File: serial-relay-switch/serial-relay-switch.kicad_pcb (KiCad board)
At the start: 2 copper layers, 41.9 x 31.8 mm, 58 parts, among them J10 Conn_01x01, J11 Conn_01x01, J12 Conn_01x01, J13 Conn_01x01, J14 Conn_01x01, J15 Conn_01x01, J16 Conn_01x01, J17 Conn_01x01, J18 Conn_01x01, J2 2501551-4, J3 Conn_01x01, J4 Conn_01x01, J5 Conn_01x01, J6 Conn_01x01, J7 Conn_01x01, J8 Conn_01x01, J9 Conn_01x01, U1 74LS166, U2 ISL8488E, U3 74LVC1G08, U4 ISL8488E

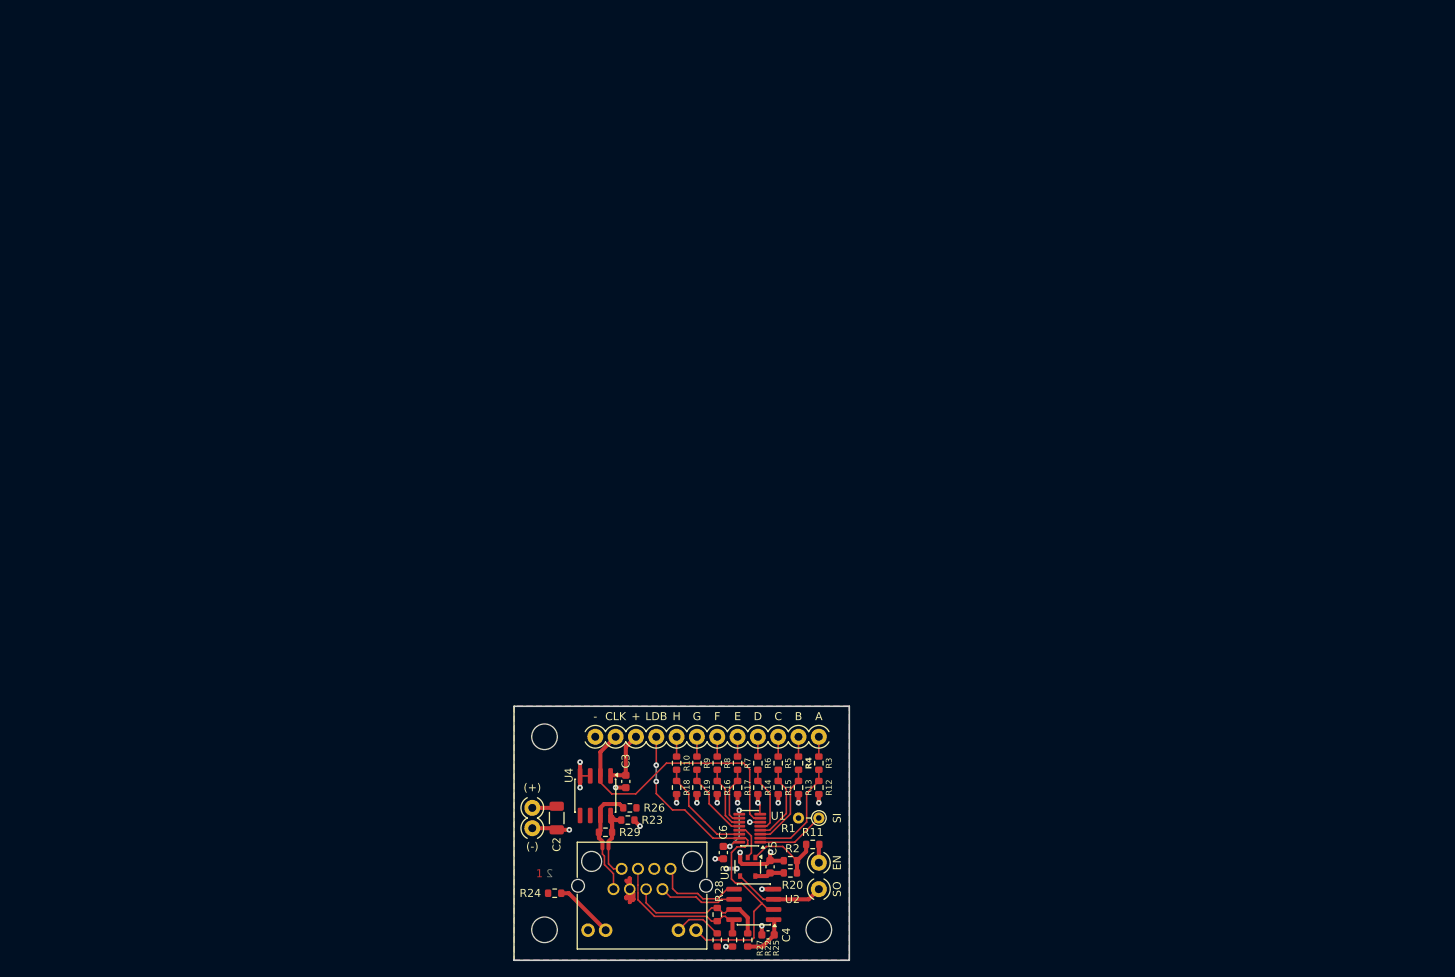
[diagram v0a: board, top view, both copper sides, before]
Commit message: [rs] Mostly complete preliminary PCB placement
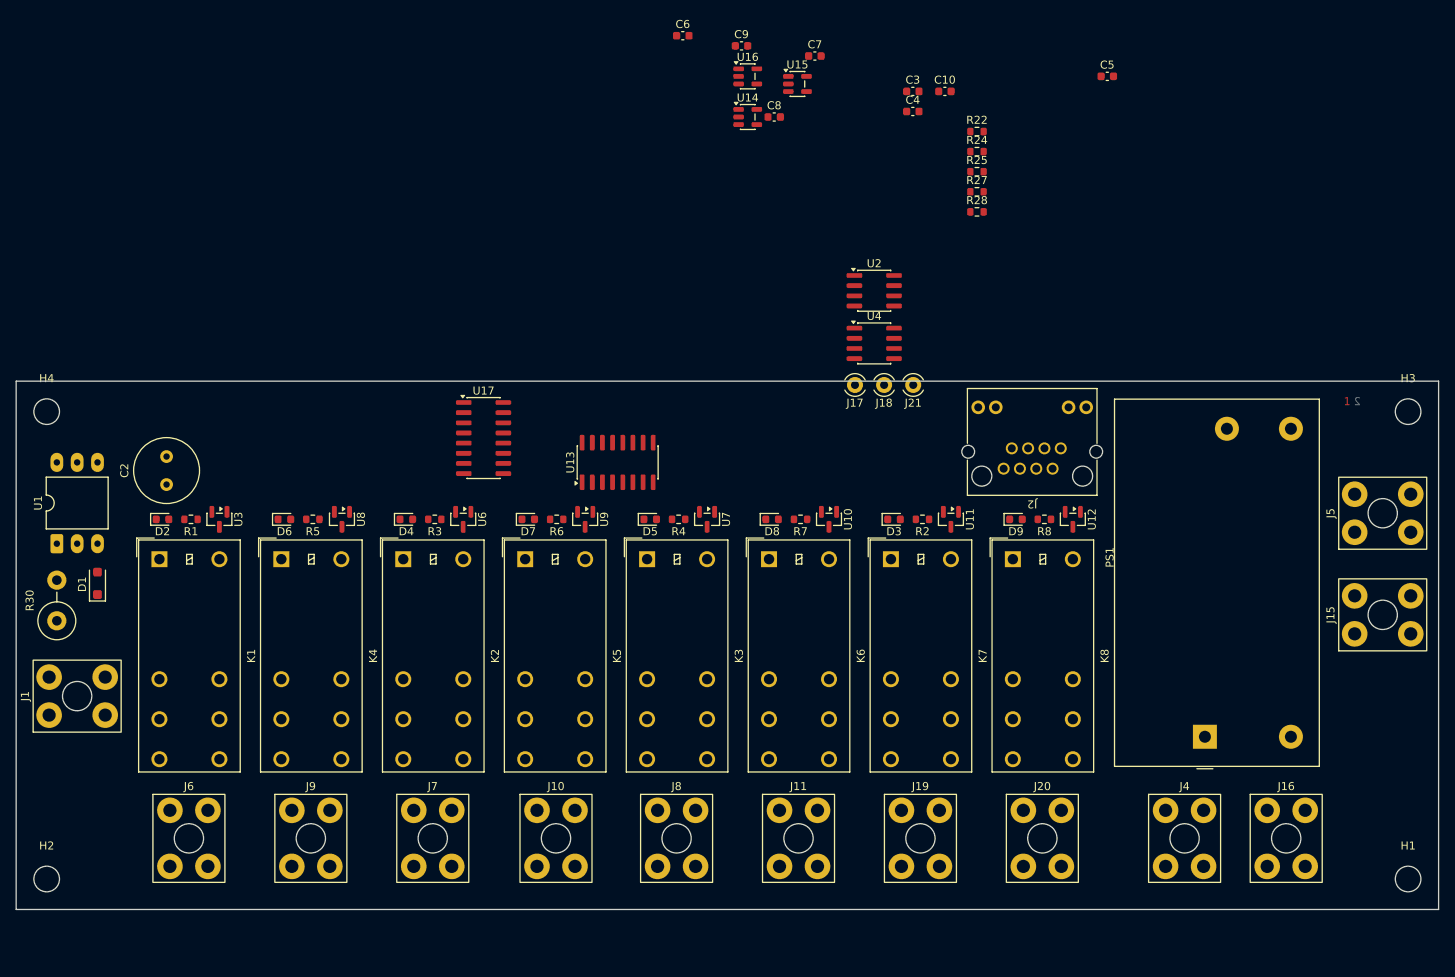
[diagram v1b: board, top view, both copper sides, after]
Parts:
- removed J12, J13, J14, J3: Conn_01x01, CUSTOM:Pin_D1.0mm
- removed R10, R11, R9: 1k, Resistor_SMD:R_0603_1608Metric
- removed R12, R13, R14, R15, R16, R17, R18, R19, R20, R23, R26: 10k, Resistor_SMD:R_0603_1608Metric
- removed R29: 120, Resistor_SMD:R_0603_1608Metric
- added C10: 0.1uF, Capacitor_SMD:C_0603_1608Metric, F.Cu at (153.9, 6.39)
- added C7: 0.1uF, Capacitor_SMD:C_0603_1608Metric, F.Cu at (137.6, 1.97)
- added C8: 0.1uF, Capacitor_SMD:C_0603_1608Metric, F.Cu at (132.5, 9.59)
- added C9: 0.1uF, Capacitor_SMD:C_0603_1608Metric, F.Cu at (128.4, 0.70)
- added D1: 1N4148, Diode_SMD:D_SOD-123F, F.Cu at (47.9, 67.9)
- added D2: LED, LED_SMD:LED_0603_1608Metric, F.Cu at (56.1, 59.9)
- added D3: LED, LED_SMD:LED_0603_1608Metric, F.Cu at (147.5, 59.9)
- added D4: LED, LED_SMD:LED_0603_1608Metric, F.Cu at (86.5, 59.9)
- added D5: LED, LED_SMD:LED_0603_1608Metric, F.Cu at (117.0, 59.9)
- added D6: LED, LED_SMD:LED_0603_1608Metric, F.Cu at (71.3, 59.9)
- added D7: LED, LED_SMD:LED_0603_1608Metric, F.Cu at (101.8, 59.9)
- added D8: LED, LED_SMD:LED_0603_1608Metric, F.Cu at (132.3, 59.9)
- added D9: LED, LED_SMD:LED_0603_1608Metric, F.Cu at (162.7, 59.9)
- added H4: MountingHole, MountingHole:MountingHole_3.2mm_M3, F.Cu at (41.6, 46.4)
- added J1: Screw_Terminal_01x01, CUSTOM:8195, F.Cu at (45.4, 82.0)
- added J19: Screw_Terminal_01x01, CUSTOM:8195, F.Cu at (150.8, 99.8)
- added J20: Screw_Terminal_01x01, CUSTOM:8195, F.Cu at (166.0, 99.8)
- added J21: Conn_01x01, CUSTOM:Pin_D1.0mm, F.Cu at (149.9, 43.1)
- added K1: G2RL-1-E, Relay_THT:Relay_SPDT_Omron_G2RL-1-E, F.Cu at (55.7, 64.9)
- added K2: G2RL-1-E, Relay_THT:Relay_SPDT_Omron_G2RL-1-E, F.Cu at (86.2, 64.9)
- added K3: G2RL-1-E, Relay_THT:Relay_SPDT_Omron_G2RL-1-E, F.Cu at (116.6, 64.9)
- added K4: G2RL-1-E, Relay_THT:Relay_SPDT_Omron_G2RL-1-E, F.Cu at (70.9, 64.9)
- added K5: G2RL-1-E, Relay_THT:Relay_SPDT_Omron_G2RL-1-E, F.Cu at (101.4, 64.9)
- added K6: G2RL-1-E, Relay_THT:Relay_SPDT_Omron_G2RL-1-E, F.Cu at (131.9, 64.9)
- added K7: G2RL-1-E, Relay_THT:Relay_SPDT_Omron_G2RL-1-E, F.Cu at (147.1, 64.9)
- added K8: G2RL-1-E, Relay_THT:Relay_SPDT_Omron_G2RL-1-E, F.Cu at (162.4, 64.9)
- added PS1: IRM-10-5, Converter_ACDC:Converter_ACDC_MeanWell_IRM-10-xx_THT, F.Cu at (186.4, 87.1)
- added R30: 100k, Resistor_THT:R_Axial_DIN0414_L11.9mm_D4.5mm_P5.08mm_Vertical, F.Cu at (42.9, 72.6)
- added U10: SZNUD3124LT1G, Package_TO_SOT_SMD:SOT-23, F.Cu at (139.4, 59.9)
- added U11: SZNUD3124LT1G, Package_TO_SOT_SMD:SOT-23, F.Cu at (154.6, 59.9)
- added U12: SZNUD3124LT1G, Package_TO_SOT_SMD:SOT-23, F.Cu at (169.8, 59.9)
- added U13: 74HCT595, Package_SO:SOIC-16_3.9x9.9mm_P1.27mm, F.Cu at (113.0, 52.8)
- added U14: 74LVC1G32, Package_TO_SOT_SMD:SOT-23-5, F.Cu at (129.2, 9.59)
- added U15: 74LVC1G08, Package_TO_SOT_SMD:SOT-23-5, F.Cu at (135.4, 5.46)
- added U16: 74LVC1G04, Package_TO_SOT_SMD:SOT-23-5, F.Cu at (129.2, 4.51)
- added U17: 74LS163, Package_SO:SOIC-16_3.9x9.9mm_P1.27mm, F.Cu at (96.2, 49.7)
- added U6: SZNUD3124LT1G, Package_TO_SOT_SMD:SOT-23, F.Cu at (93.7, 59.9)
- added U7: SZNUD3124LT1G, Package_TO_SOT_SMD:SOT-23, F.Cu at (124.1, 59.9)
- added U8: SZNUD3124LT1G, Package_TO_SOT_SMD:SOT-23, F.Cu at (78.5, 59.9)
- added U9: SZNUD3124LT1G, Package_TO_SOT_SMD:SOT-23, F.Cu at (108.9, 59.9)
- C2: footprint Capacitor_SMD:C_1206_3216Metric -> Capacitor_THT:C_Radial_D8.0mm_H7.0mm_P3.50mm
- J10, J11, J15, J16, J4, J5, J6, J7, J8, J9: value Conn_01x01 -> Screw_Terminal_01x01; footprint CUSTOM:Pin_D1.0mm -> CUSTOM:8195
- R1: value 10k -> 1k; footprint Resistor_THT:R_Axial_DIN0204_L3.6mm_D1.6mm_P2.54mm_Vertical -> Resistor_SMD:R_0603_1608Metric
- R2: value 10k -> 1k
- U1: value 74LS166 -> H11L1; footprint Package_SO:Texas_DYY0016A_TSOT-23-16_2x4.2mm_P0.5mm -> Package_DIP:DIP-6_W10.16mm_LongPads
- U3: value 74LVC1G08 -> SZNUD3124LT1G; footprint Package_SO:TSOP-5_1.65x3.05mm_P0.95mm -> Package_TO_SOT_SMD:SOT-23
- moved H3 125.9 mm to (211.8, 46.4)
- moved LAY1 116.9 mm to (204.1, 46.4)
- moved H1 109.4 mm to (211.8, 104.8)
- moved J15 109.0 mm to (208.6, 71.8)
- moved C5 107.4 mm to (174.2, 4.51), turned to 0 degrees
- moved R24 106.7 mm to (157.9, 13.9), turned to 0 degrees
- moved R22 105.6 mm to (157.9, 11.4), turned to 0 degrees
- moved C4 104.5 mm to (149.8, 8.90), turned to 0 degrees
- moved C6 102.2 mm to (121.1, -0.57), turned to 0 degrees
- moved R25 100.2 mm to (157.9, 16.4), turned to 0 degrees
- moved R27 99.0 mm to (157.9, 18.9), turned to 0 degrees
- moved H2 96.7 mm to (41.6, 104.8)
- moved J16 94.2 mm to (196.5, 99.8), turned to 0 degrees
- moved R28 93.6 mm to (157.9, 21.4), turned to 0 degrees
- moved U1 93.6 mm to (42.9, 62.9), turned to 90 degrees
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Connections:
- J10 pad 1: Net-(J10-Pin_1) -> /OUT_D
- J11 pad 1: Net-(J11-Pin_1) -> /OUT_F
- J15 pad 1: +5V -> GND
- J16 pad 1: GND -> /NEUTRAL
- J17 pad 1: /LOADB -> /SCAN_IN
- J2 pad 12: /LOADB -> GND
- J2 pad 7: /SO_N -> /SI_N
- J2 pad 8: /SO_P -> /SI_P
- J4 pad 1: Net-(J4-Pin_1) -> /NEUTRAL
- J5 pad 1: Net-(J5-Pin_1) -> GND
- J6 pad 1: Net-(J6-Pin_1) -> /OUT_A
- J7 pad 1: Net-(J7-Pin_1) -> /OUT_C
- J8 pad 1: Net-(J8-Pin_1) -> /OUT_E
- J9 pad 1: Net-(J9-Pin_1) -> /OUT_B
- R1 pad 1: /SCAN_IN -> /CTL_A
- R1 pad 2: GND -> Net-(D2-A)
- R2 pad 1: Net-(R11-Pad2) -> /CTL_G
- R2 pad 2: GND -> Net-(D3-A)
- R22 pad 2: /LD_P -> /SI_P
- R25 pad 1: /LD_N -> /SI_N
- R27 pad 2: +5V -> /COUNT_RCO
- R28 pad 1: /LD_N -> /SI_N
- R28 pad 2: /LD_P -> /SI_P
- R3 pad 1: Net-(J3-Pin_1) -> /CTL_C
- R3 pad 2: /IN_A -> Net-(D4-A)
- R4 pad 1: Net-(J4-Pin_1) -> /CTL_E
- R4 pad 2: /IN_B -> Net-(D5-A)
- R5 pad 1: Net-(J5-Pin_1) -> /CTL_B
- R5 pad 2: /IN_C -> Net-(D6-A)
- R6 pad 1: Net-(J6-Pin_1) -> /CTL_D
- R6 pad 2: /IN_D -> Net-(D7-A)
- R7 pad 1: Net-(J7-Pin_1) -> /CTL_F
- R7 pad 2: /IN_E -> Net-(D8-A)
- R8 pad 1: Net-(J8-Pin_1) -> /CTL_H
- R8 pad 2: /IN_F -> Net-(D9-A)
- U1 pad 1: /SCAN_IN -> Net-(D1-K)
- U1 pad 2: /IN_A -> /NEUTRAL
- U1 pad 3: /IN_B -> unconnected-(U1-Pad3)
- U1 pad 4: /IN_C -> /CLK
- U1 pad 5: /IN_D -> GND
- U1 pad 6: GND -> +5V
- U2 pad 2: /LOADB -> /SCAN_IN
- U2 pad 3: /SCAN_OUT -> /LOAD
- U2 pad 5: /SO_P -> /LD_P
- U2 pad 6: /SO_N -> /LD_N
- U2 pad 7: /LD_N -> /SI_N
- U2 pad 8: /LD_P -> /SI_P
- U3 pad 1: Net-(R11-Pad2) -> /CTL_A
- U3 pad 2: Net-(U1-Qh) -> GND
- U3 pad 3: GND -> Net-(K1-PadA2)
- U4 pad 2: /CLK -> unconnected-(U4-RO-Pad2)
- U4 pad 3: GND -> /CLK
- U4 pad 5: unconnected-(U4-Y-Pad5) -> /CLK_P
- U4 pad 6: unconnected-(U4-Z-Pad6) -> /CLK_N
- U4 pad 7: /CLK_N -> unconnected-(U4-B-Pad7)
- U4 pad 8: /CLK_P -> unconnected-(U4-A-Pad8)
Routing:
- net /LOADB: track 46.6 -> 0.00 mm, vias 2 -> 0
- net +5V: track 38.0 -> 0.00 mm, vias 4 -> 0
- net GND: track 35.5 -> 0.00 mm, vias 20 -> 0
- net /CLK: track 34.8 -> 0.00 mm
- net /LD_P: track 19.2 -> 0.00 mm
- net /LD_N: track 18.0 -> 0.00 mm
- net /CLK_N: track 14.3 -> 0.00 mm
- net /IN_A: track 13.8 -> 0.00 mm
- net /IN_H: track 13.1 -> 0.00 mm
- net /CLK_P: track 12.0 -> 0.00 mm
- net /SCAN_OUT: track 11.6 -> 0.00 mm
- net /SO_P: track 11.3 -> 0.00 mm
- net /IN_B: track 10.8 -> 0.00 mm
- net Net-(R11-Pad2): track 10.5 -> 0.00 mm
- net /IN_C: track 10.0 -> 0.00 mm
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- removed copper zone on F.Cu, net +5V
- removed copper zone on B.Cu, net GND
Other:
- board size 41.9 x 31.8 mm -> 177.8 x 66 mm
- board text removed: "(+)"
- board text removed: "(-)"
- board text removed: "+"
- board text removed: "-"
- board text removed: "A"
- board text removed: "B"
- board text removed: "C"
- board text removed: "CLK"
- board text removed: "D"
- board text removed: "E"
- board text removed: "EN"
- board text removed: "F"
- board text removed: "G"
- board text removed: "H"
- board text removed: "LDB"
- board text removed: "SI"
- board text removed: "SO"
